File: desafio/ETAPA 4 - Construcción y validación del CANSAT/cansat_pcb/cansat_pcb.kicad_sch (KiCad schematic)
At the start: 15 parts, among them J1 HEADER, U1 MPU-6050, U2 LDO-3.3

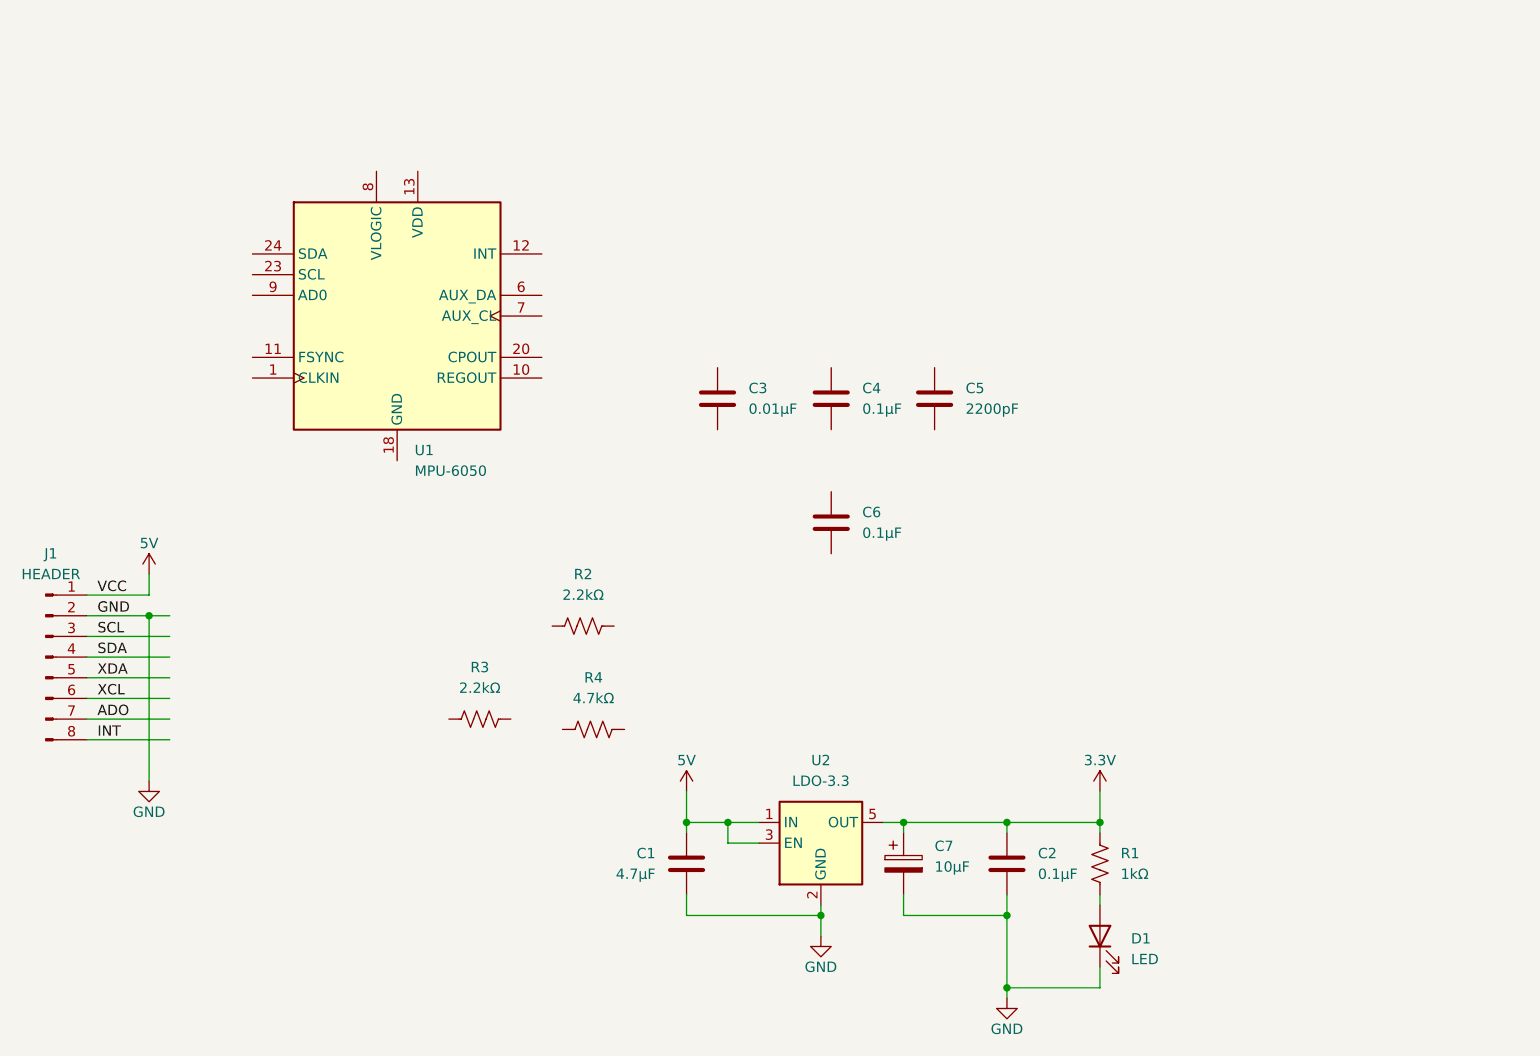
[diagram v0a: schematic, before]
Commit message: update pcb
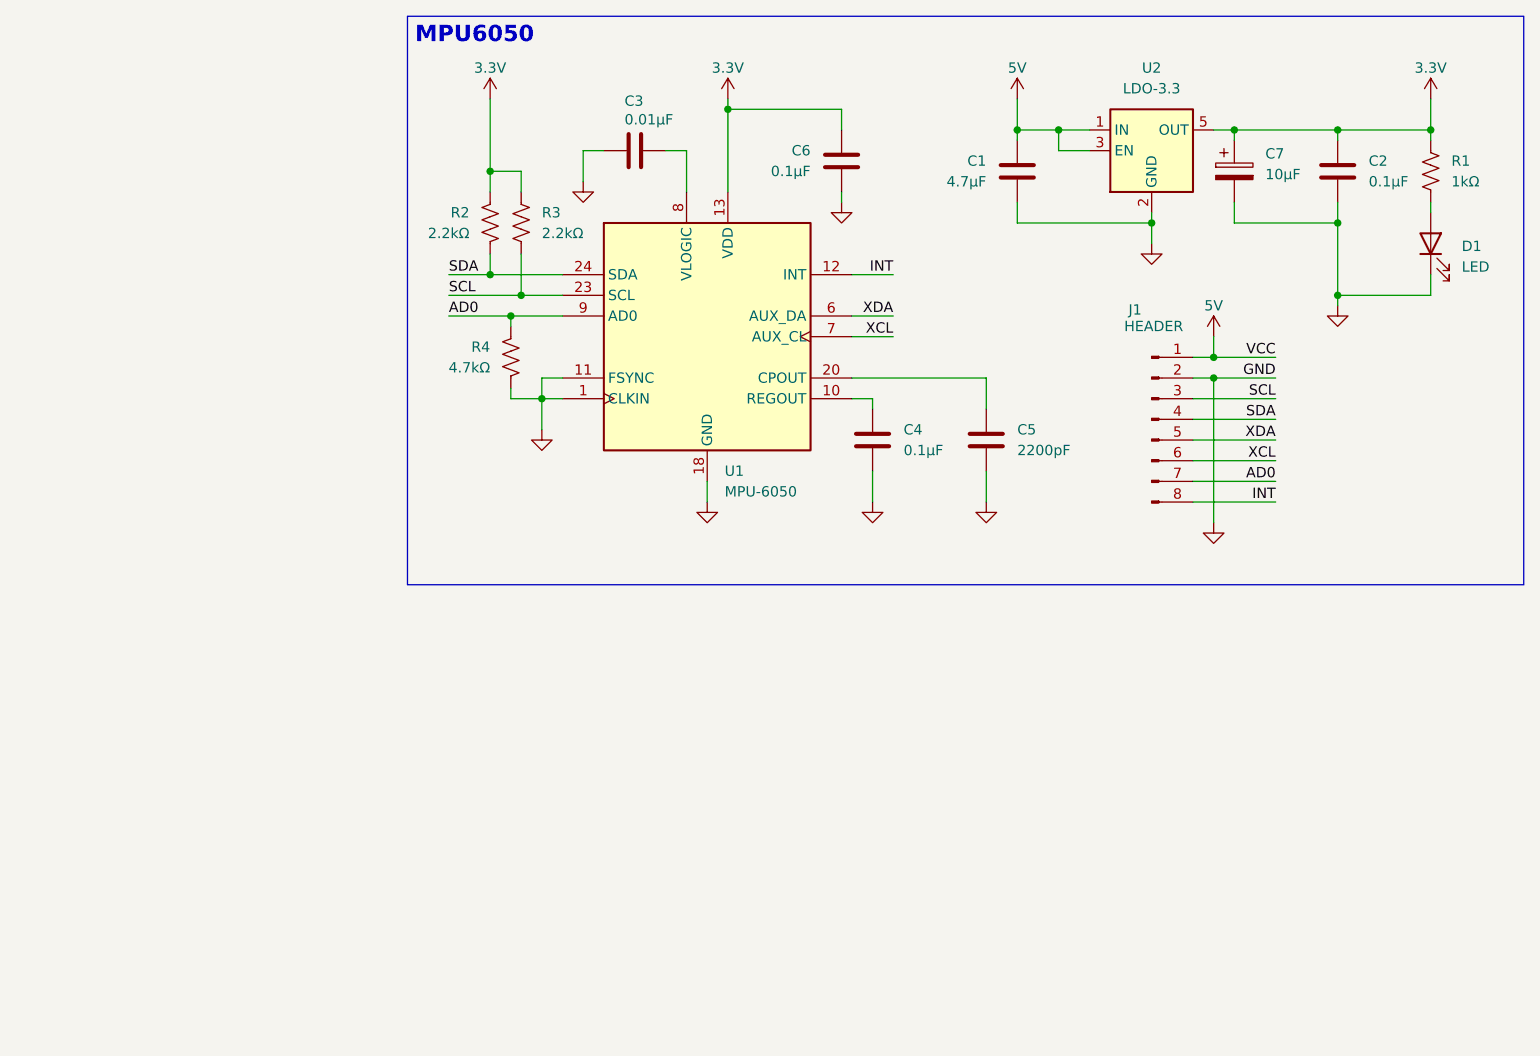
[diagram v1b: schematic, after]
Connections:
- net ADO is gone; now on net AD0: J1.7 (Pin_7)
- net 3.3V: now also C6.1, R2.1, R3.2, U1.13 (VDD)
- net GND: now also C3.2, C4.2, C5.2, C6.2, R4.2, U1.1 (CLKIN), U1.11 (FSYNC), U1.18 (GND)
- net INT: now also U1.12 (INT)
- net SCL: now also R3.1, U1.23 (SCL)
- net SDA: now also R2.2, U1.24 (SDA)
- net XCL: now also U1.7 (AUX_CL)
- net XDA: now also U1.6 (AUX_DA)
- net at U1.10 (REGOUT): now also C4.1
- net at U1.20 (CPOUT): now also C5.1
- net at U1.8 (VLOGIC): now also C3.1
- net AD0: now reaches U1.9 (AD0)
- net AD0: now also R4.1
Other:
- moved on the sheet: C1, C2, C3, C4, C5, C6, C7, D1, J1, R1, R2, R3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
